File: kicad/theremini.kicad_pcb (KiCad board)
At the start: 2 copper layers, 60 x 54.5 mm, 6 parts, among them U1 NAU88C22YG, U2 VL53L0CXV0DH/1, U4 VL53L0CXV0DH/1, U5 KLJ-01304T-08R07W, U6 PJ-327C-4A, U7 STM32L432KBU6TR

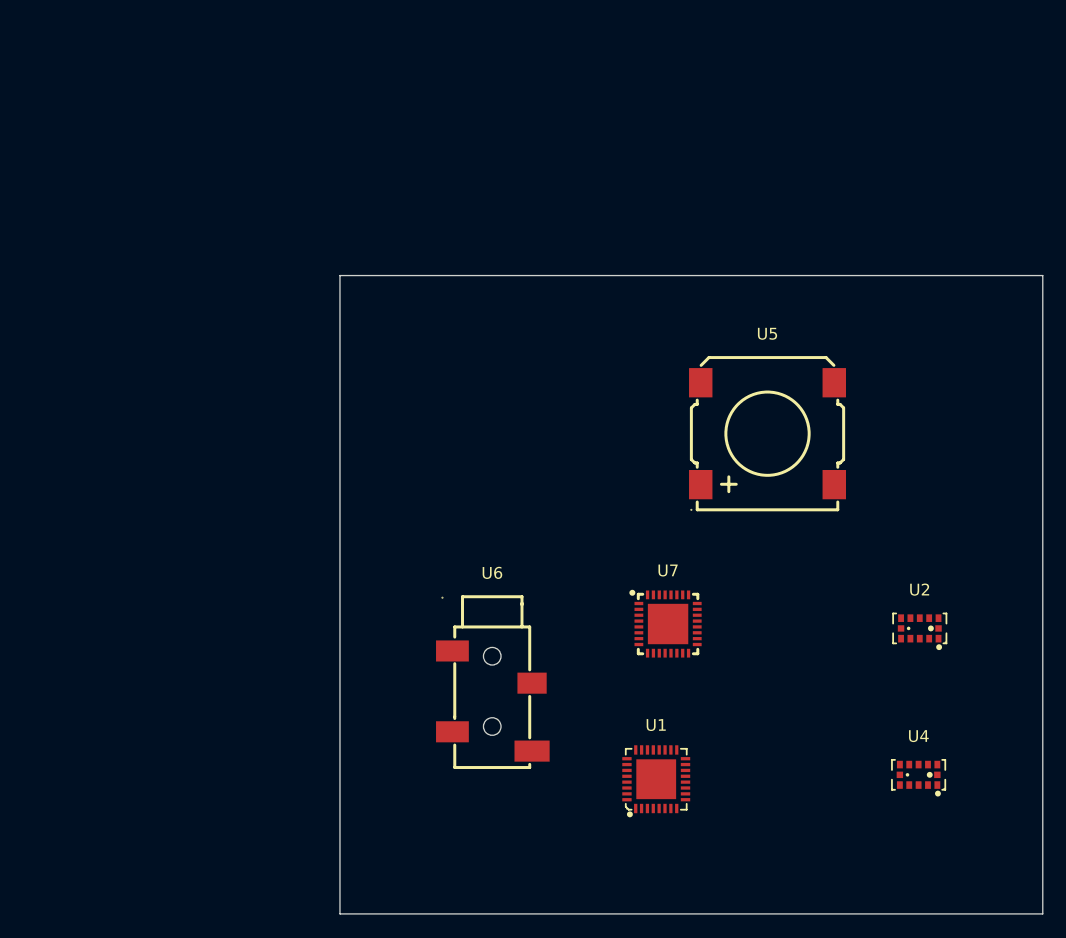
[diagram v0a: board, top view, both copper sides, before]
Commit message: Connected things
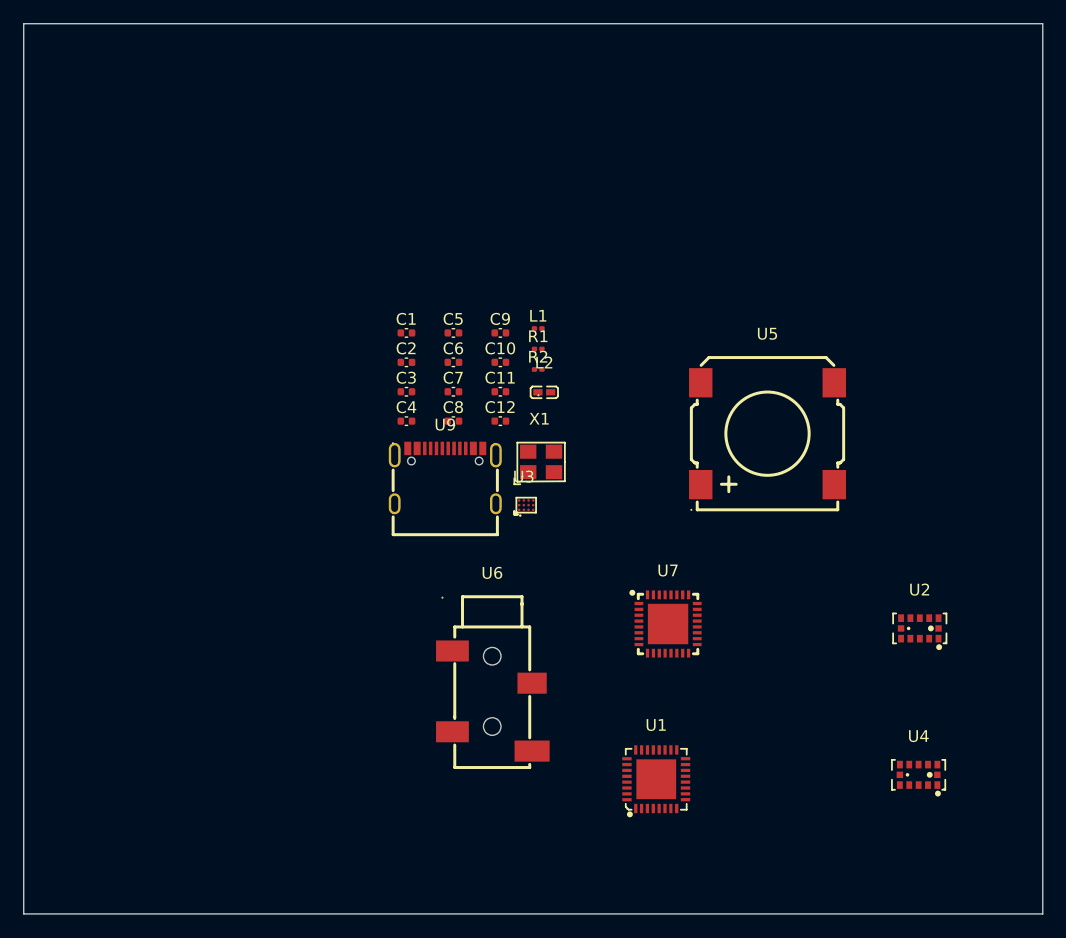
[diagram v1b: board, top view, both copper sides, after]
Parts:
- added C1: 10u, Capacitor_SMD:C_0402_1005Metric, F.Cu at (100.7, 85.9)
- added C10: 100n, Capacitor_SMD:C_0402_1005Metric, F.Cu at (108.7, 88.4)
- added C11: 100n, Capacitor_SMD:C_0402_1005Metric, F.Cu at (108.7, 90.9)
- added C12: 15p, Capacitor_SMD:C_0402_1005Metric, F.Cu at (108.7, 93.4)
- added C2: 10u, Capacitor_SMD:C_0402_1005Metric, F.Cu at (100.7, 88.4)
- added C3: 10u, Capacitor_SMD:C_0402_1005Metric, F.Cu at (100.7, 90.9)
- added C4: 1n, Capacitor_SMD:C_0402_1005Metric, F.Cu at (100.7, 93.4)
- added C5: 4u7, Capacitor_SMD:C_0402_1005Metric, F.Cu at (104.7, 85.9)
- added C6: 100n, Capacitor_SMD:C_0402_1005Metric, F.Cu at (104.7, 88.4)
- added C7: 100n, Capacitor_SMD:C_0402_1005Metric, F.Cu at (104.7, 90.9)
- added C8: 10n, Capacitor_SMD:C_0402_1005Metric, F.Cu at (104.7, 93.4)
- added C9: 1u, Capacitor_SMD:C_0402_1005Metric, F.Cu at (108.7, 85.9)
- added L1: 1.5u, Inductor_SMD:L_0201_0603Metric, F.Cu at (111.9, 85.5)
- added L2: BLM15AG601SN1D, BLM15AG601SN1D:L0402, F.Cu at (112.4, 91.0)
- added R1: 1M, Resistor_SMD:R_0201_0603Metric, F.Cu at (111.9, 87.3)
- added R2: 10k, Resistor_SMD:R_0201_0603Metric, F.Cu at (111.9, 89.0)
- added U3: TPS63051YFFR, TPS63051YFFR:DSBGA-12_L1.6-W1.2-R3-C4-P0.40-BL, F.Cu at (110.9, 100.6)
- added U9: TYPE-C16PIN, TYPE-C16PIN:USB-C-SMD_TYPE-C16PIN, F.Cu at (104.0, 98.1)
- added X1: OT32258MJBA4SL, OT32258MJBA4SL:OSC-SMD_4P-L3.2-W2.5-BL, F.Cu at (112.2, 96.9)
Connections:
- U7 pad 1: unconnected-(U7-VDD-Pad1) -> +3.3V
- U7 pad 17: unconnected-(U7-VDD-Pad17) -> +3.3V
- U7 pad 31: unconnected-(U7-PH3/BOOT0-Pad31) -> Net-(U7-PH3/BOOT0)
- U7 pad 32: unconnected-(U7-VSS-Pad32) -> GND
- U7 pad 4: unconnected-(U7-NRST-Pad4) -> NRST
- U7 pad 5: unconnected-(U7-VDDA/VREF+-Pad5) -> VDDA
- U7 pad 6: unconnected-(U7-PA0/CK_IN-Pad6) -> XTAL OUT
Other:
- board size 60 x 54.5 mm -> 87 x 76 mm
